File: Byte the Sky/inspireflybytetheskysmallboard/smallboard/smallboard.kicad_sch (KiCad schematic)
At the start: 18 parts, among them IC1 N34TS04MT3ETG, IC2 IIS2MDCTR, J1 Conn_01x07_Pin, U2 LSM6DSV, U3 OPA381

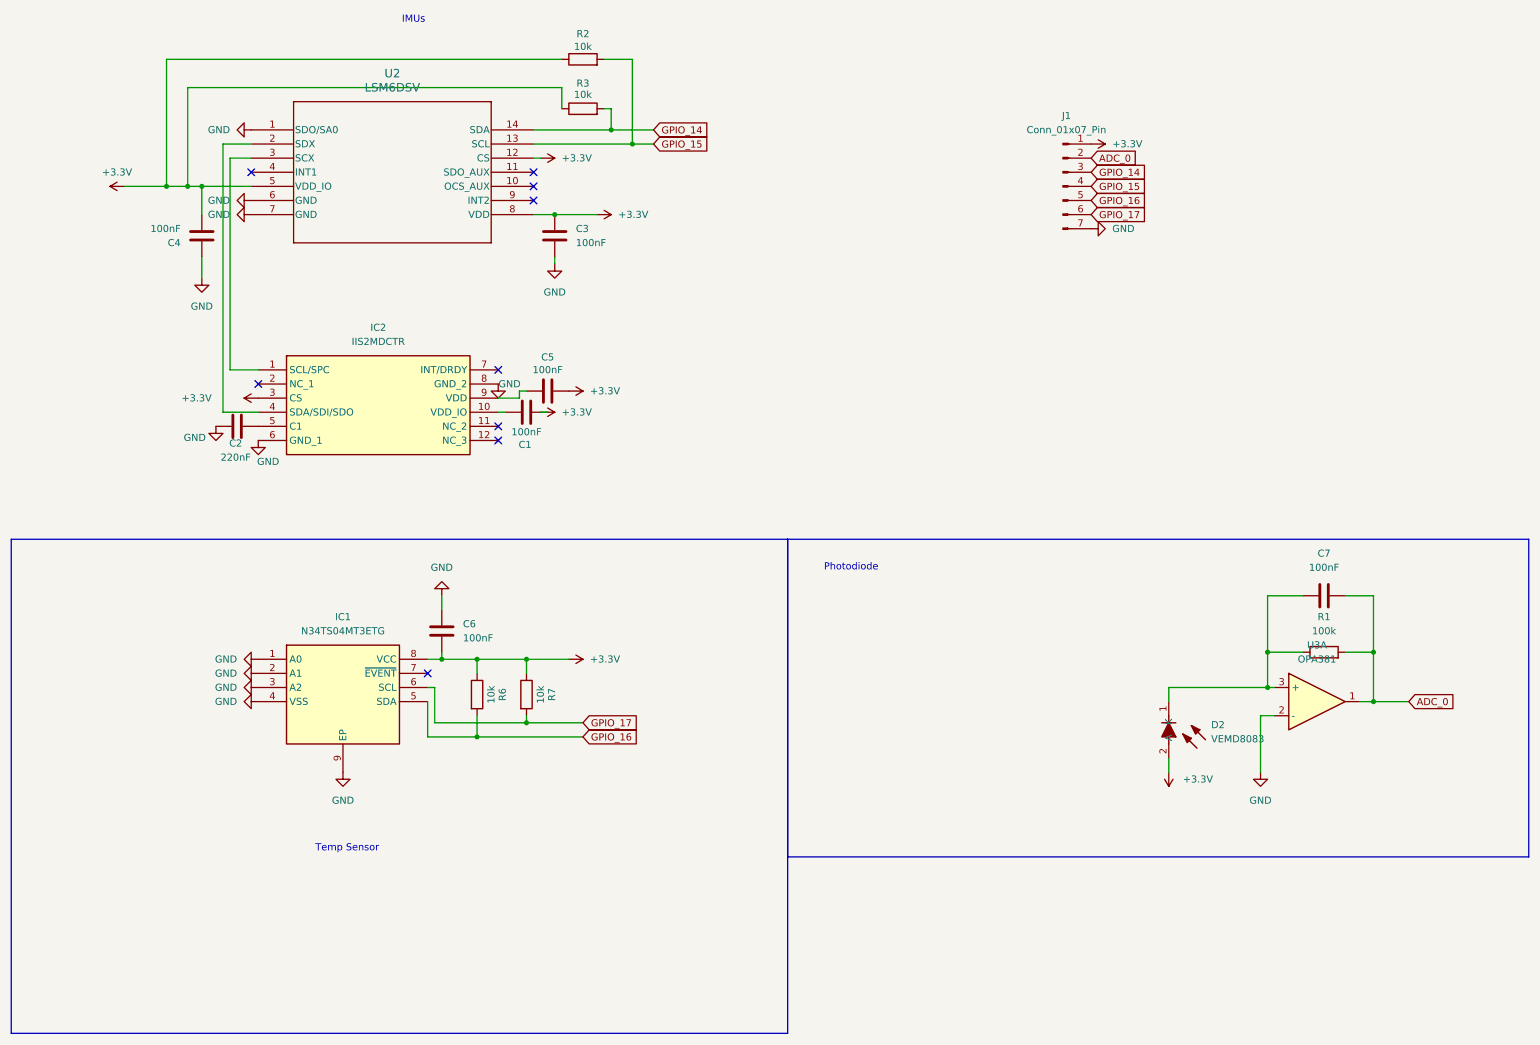
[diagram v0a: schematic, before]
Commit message: Add files via upload
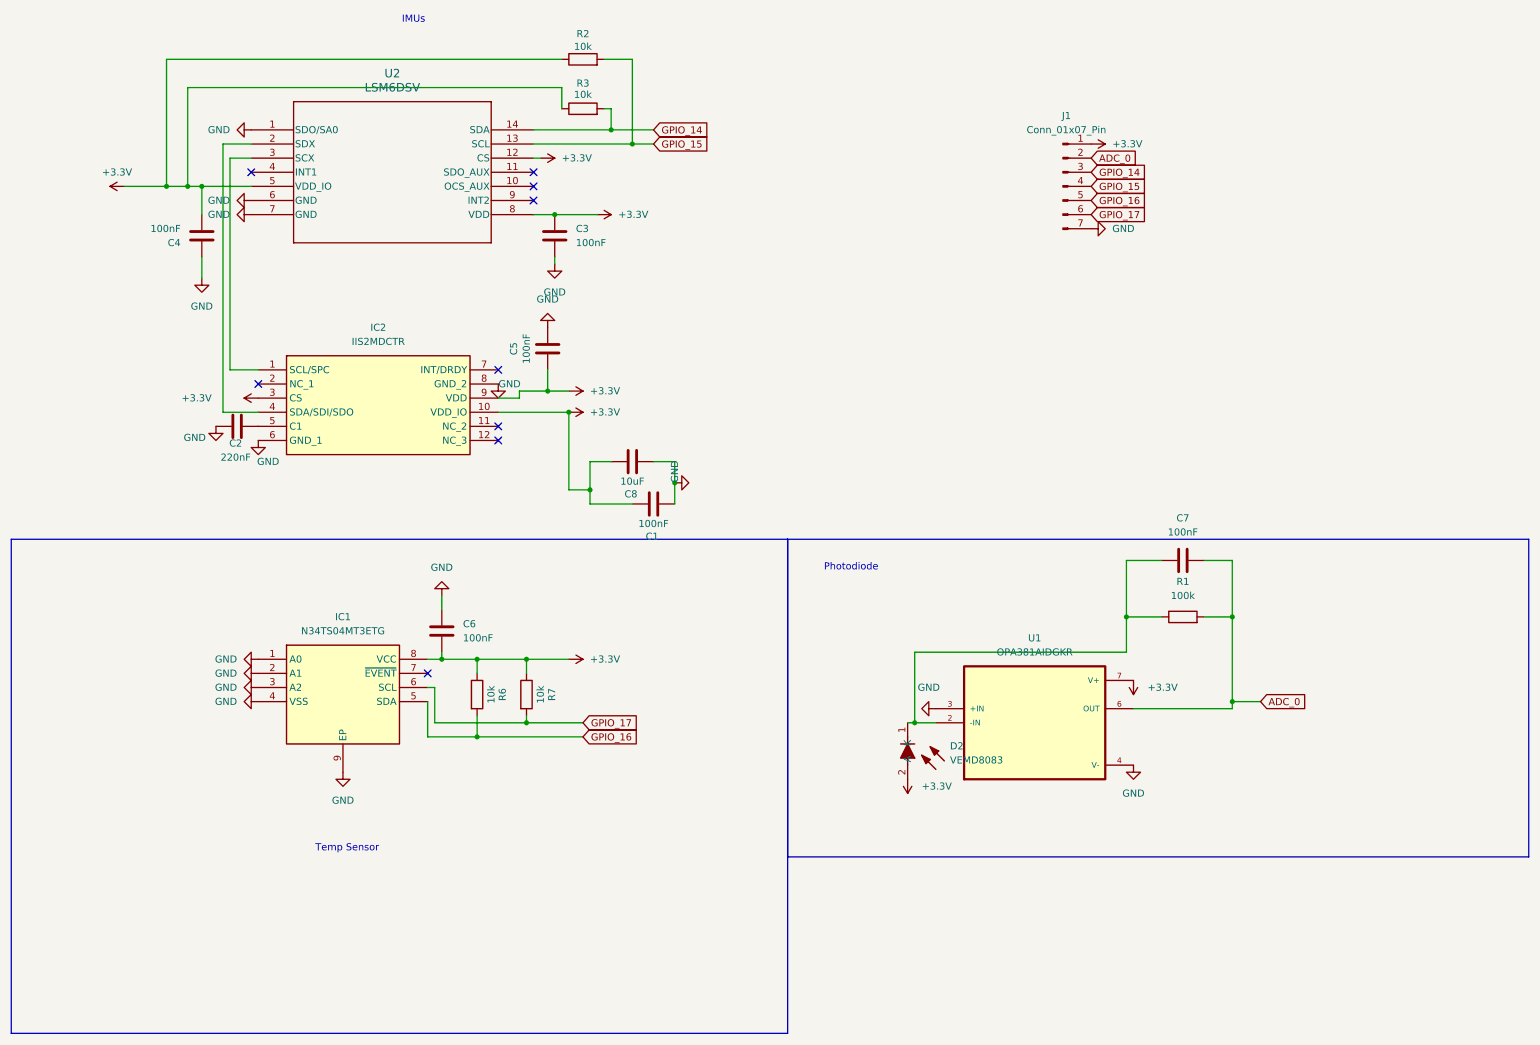
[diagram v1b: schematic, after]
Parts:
- removed U3: OPA381, OPA381:OPA381 Amplifier, symbol Device:Opamp_Dual
- added C8: 10uF, Capacitor_SMD:C_0402_1005Metric_Pad0.74x0.62mm_HandSolder, symbol Device:C
- added U1: OPA381AIDGKR, OPA381AIDGKR:SOP65P490X110-8N, symbol OPA381AIDGKR:OPA381AIDGKR
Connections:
- net +3.3V: now also C1.1, C5.1, IC2.10 (VDD_IO), IC2.9 (VDD), C8.1, U1.7 (V+); no longer C1.2, C5.2
- net ADC_0: now also U1.6 (OUT)
- net GND: now also C1.2, C5.2, C8.2, U1.3 (+IN), U1.4 (V-)
- net at C7.1, D2.1 (K), R1.1: now also U1.2 (-IN)
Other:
- moved on the sheet: C1, C5, C7, D2, R1
